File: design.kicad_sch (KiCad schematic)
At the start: 4 parts, among them J1 BM04B-SRSS-TB_LF__SN_, SW1 SW_Push, SW2 SW_Push

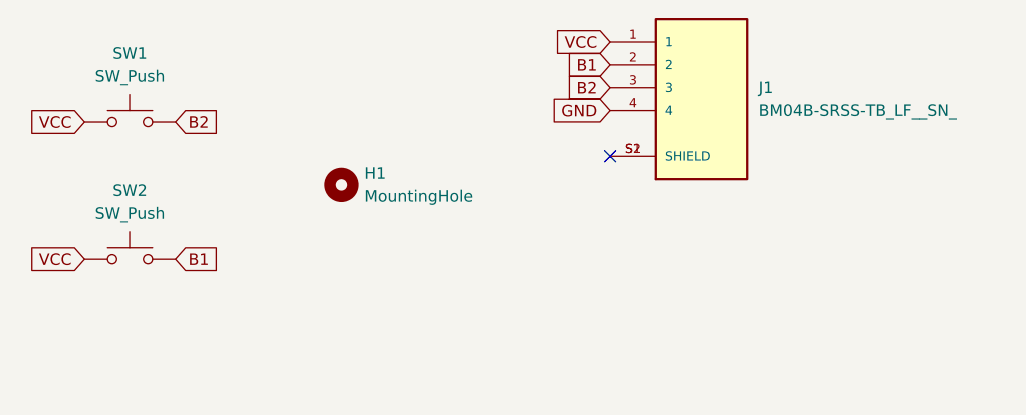
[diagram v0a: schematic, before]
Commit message: update
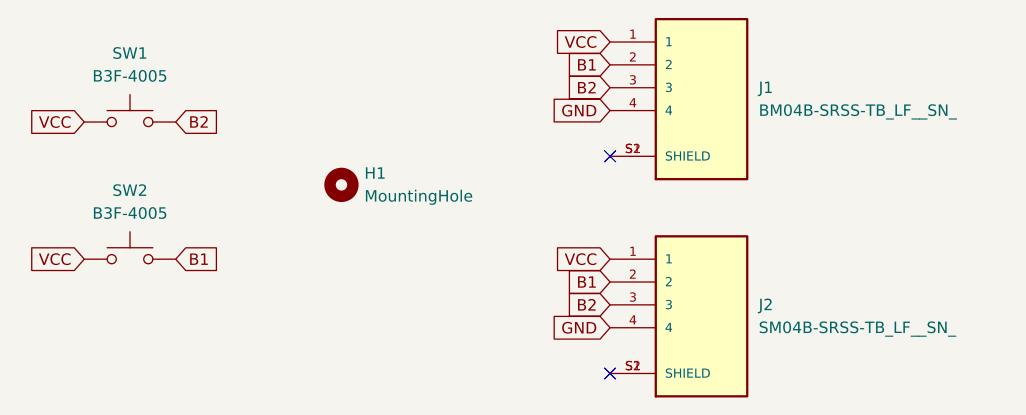
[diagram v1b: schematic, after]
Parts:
- added J2: SM04B-SRSS-TB_LF__SN_, Connector_JST:JST_SH_SM04B-SRSS-TB_1x04-1MP_P1.00mm_Horizontal, symbol Snapeda:BM04B-SRSS-TB_LF__SN_
- SW1, SW2: value SW_Push -> B3F-4005
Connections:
- net B1: now also J2.2
- net B2: now also J2.3
- net GND: now also J2.4
- net VCC: now also J2.1
- new net: J2.S1 (SHIELD), J2.S2 (SHIELD)
- no-connect marks 1 -> 2
